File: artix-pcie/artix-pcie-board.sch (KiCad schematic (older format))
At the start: 0 parts

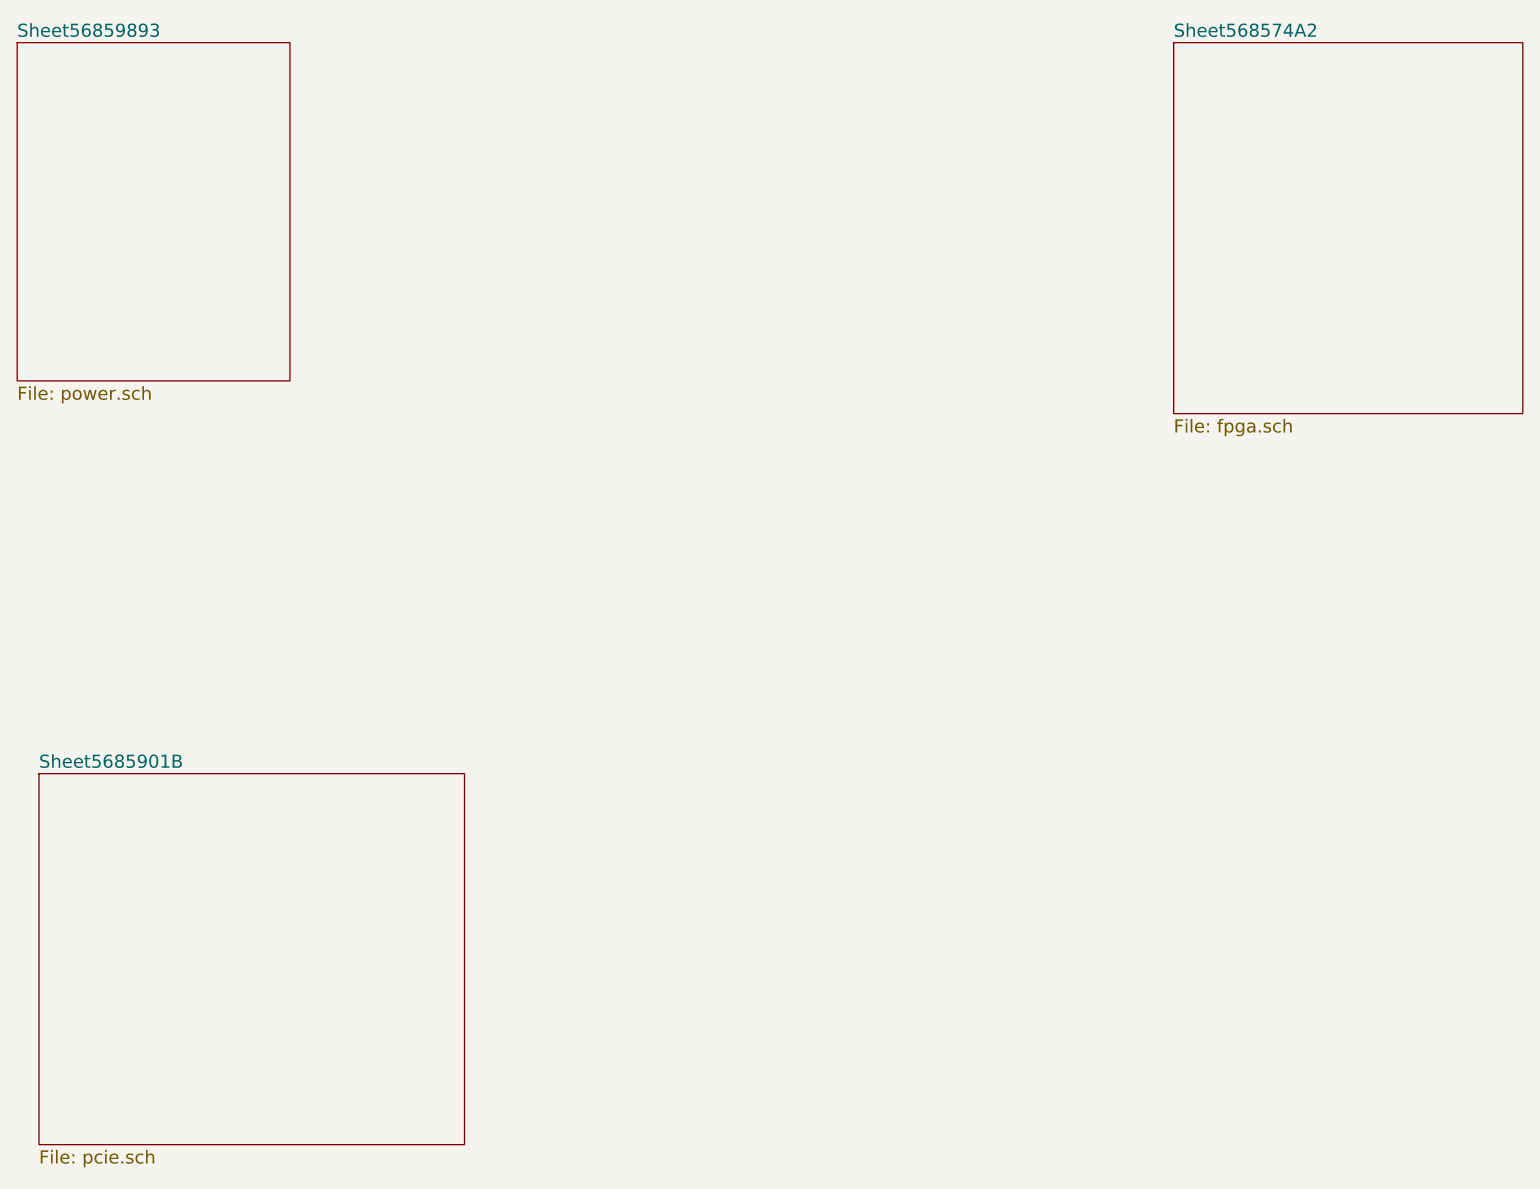
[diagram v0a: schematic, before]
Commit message: working the hierarchy
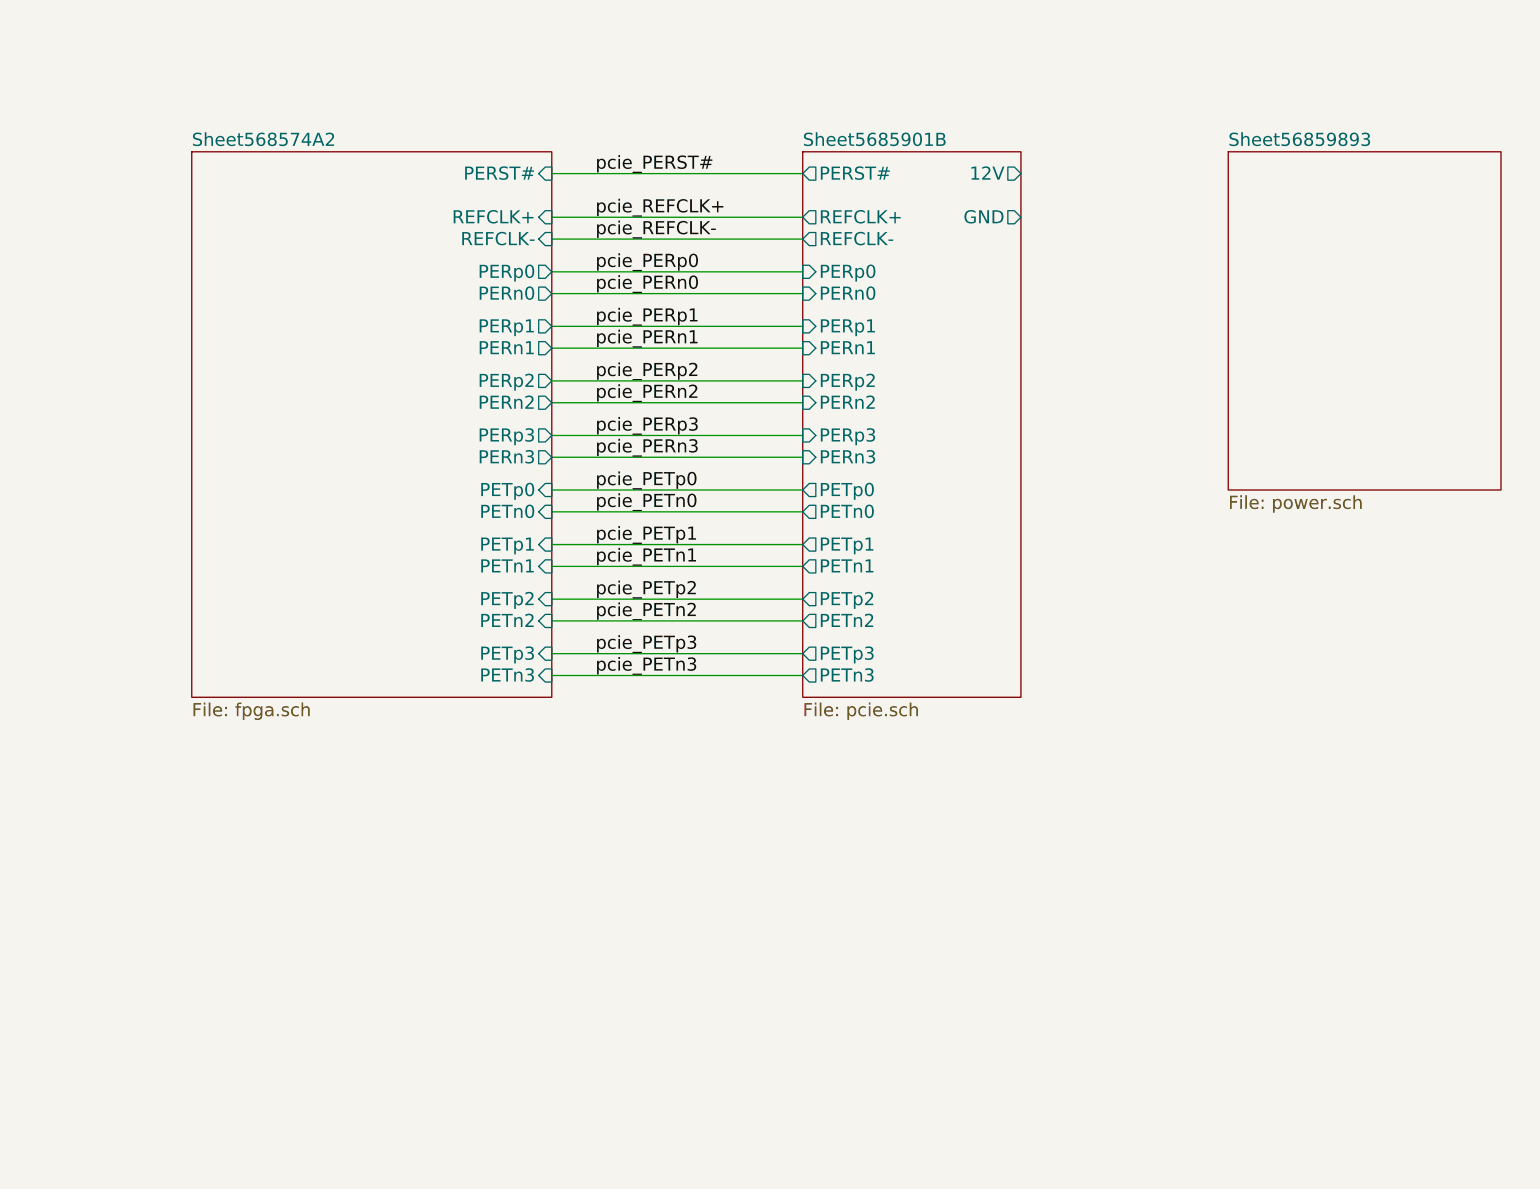
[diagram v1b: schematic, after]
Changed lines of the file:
@@
 EESchema Schematic File Version 2
+LIBS:artix-pcie-board-rescue
 LIBS:TOFE
 LIBS:xilinx7
@@
 $EndDescr
 $Sheet
-S 7650 1800 1600 1700
+S 3150 2300 1650 2500
 U 568574A3
 F0 "Sheet568574A2" 60
 F1 "fpga.sch" 60
+F2 "PETp0" I R 4800 3850 60
+F3 "PETn0" I R 4800 3950 60
+F4 "PETp1" I R 4800 4100 60
+F5 "PETn1" I R 4800 4200 60
+F6 "PETp2" I R 4800 4350 60
+F7 "PETn2" I R 4800 4450 60
+F8 "PETp3" I R 4800 4600 60
+F9 "PETn3" I R 4800 4700 60
+F10 "REFCLK+" I R 4800 2600 60
+F11 "REFCLK-" I R 4800 2700 60
+F12 "PERp0" O R 4800 2850 60
+F13 "PERn0" O R 4800 2950 60
+F14 "PERp1" O R 4800 3100 60
+F15 "PERn1" O R 4800 3200 60
+F16 "PERp2" O R 4800 3350 60
+F17 "PERn2" O R 4800 3450 60
+F18 "PERp3" O R 4800 3600 60
+F19 "PERn3" O R 4800 3700 60
+F20 "PERST#" I R 4800 2400 60
 $EndSheet
 $Sheet
-S 2450 5150 1950 1700
+S 5950 2300 1000 2500
 U 5685901C
 F0 "Sheet5685901B" 60
 F1 "pcie.sch" 60
+F2 "12V" O R 6950 2400 60
+F3 "GND" O R 6950 2600 60
+F4 "REFCLK+" O L 5950 2600 60
+F5 "REFCLK-" O L 5950 2700 60
+F6 "PETp0" O L 5950 3850 60
+F7 "PETn0" O L 5950 3950 60
+F8 "PETp1" O L 5950 4100 60
+F9 "PETn1" O L 5950 4200 60
+F10 "PETp2" O L 5950 4350 60
+F11 "PETn2" O L 5950 4450 60
+F12 "PETp3" O L 5950 4600 60
+F13 "PETn3" O L 5950 4700 60
+F14 "PERp0" I L 5950 2850 60
+F15 "PERn0" I L 5950 2950 60
+F16 "PERp1" I L 5950 3100 60
+F17 "PERn1" I L 5950 3200 60
+F18 "PERp2" I L 5950 3350 60
+F19 "PERn2" I L 5950 3450 60
+F20 "PERp3" I L 5950 3600 60
+F21 "PERn3" I L 5950 3700 60
+F22 "PERST#" O L 5950 2400 60
 $EndSheet
 $Sheet
-S 2350 1800 1250 1550
+S 7900 2300 1250 1550
 U 56859894
 F0 "Sheet56859893" 60
 F1 "power.sch" 60
 $EndSheet
+Wire Wire Line
+	4800 2400 5950 2400
+Wire Wire Line
+	5950 2600 4800 2600
+Wire Wire Line
+	4800 2700 5950 2700
+Wire Wire Line
+	5950 2850 4800 2850
+Wire Wire Line
+	4800 2950 5950 2950
+Wire Wire Line
+	5950 3100 4800 3100
+Wire Wire Line
+	4800 3200 5950 3200
+Wire Wire Line
+	4800 3350 5950 3350
+Wire Wire Line
+	5950 3450 4800 3450
+Wire Wire Line
+	4800 3600 5950 3600
+Wire Wire Line
+	5950 3700 4800 3700
+Wire Wire Line
+	4800 3850 5950 3850
+Wire Wire Line
+	5950 3950 4800 3950
+Wire Wire Line
+	4800 4100 5950 4100
+Wire Wire Line
+	5950 4200 4800 4200
+Wire Wire Line
+	4800 4350 5950 4350
+Wire Wire Line
+	5950 4450 4800 4450
+Wire Wire Line
+	4800 4600 5950 4600
+Wire Wire Line
+	5950 4700 4800 4700
+Text Label 5000 2400 0    60   ~ 0
+pcie_PERST#
+Text Label 5000 2600 0    60   ~ 0
+pcie_REFCLK+
+Text Label 5000 2700 0    60   ~ 0
+pcie_REFCLK-
+Text Label 5000 2850 0    60   ~ 0
+pcie_PERp0
+Text Label 5000 2950 0    60   ~ 0
+pcie_PERn0
+Text Label 5000 3100 0    60   ~ 0
+pcie_PERp1
+Text Label 5000 3350 0    60   ~ 0
+pcie_PERp2
+Text Label 5000 3600 0    60   ~ 0
+pcie_PERp3
+Text Label 5000 3850 0    60   ~ 0
+pcie_PETp0
+Text Label 5000 3950 0    60   ~ 0
+pcie_PETn0
+Text Label 5000 3200 0    60   ~ 0
+pcie_PERn1
+Text Label 5000 3450 0    60   ~ 0
+pcie_PERn2
+Text Label 5000 3700 0    60   ~ 0
+pcie_PERn3
+Text Label 5000 4100 0    60   ~ 0
+pcie_PETp1
+Text Label 5000 4350 0    60   ~ 0
+pcie_PETp2
+Text Label 5000 4600 0    60   ~ 0
+pcie_PETp3
+Text Label 5000 4200 0    60   ~ 0
+pcie_PETn1
+Text Label 5000 4450 0    60   ~ 0
+pcie_PETn2
+Text Label 5000 4700 0    60   ~ 0
+pcie_PETn3
 $EndSCHEMATC
